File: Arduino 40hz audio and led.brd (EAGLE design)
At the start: 79.2 x 83.2 mm, 28 parts, among them IC1 LM7805, IC2 IRL-Z44N, IC3 LM741

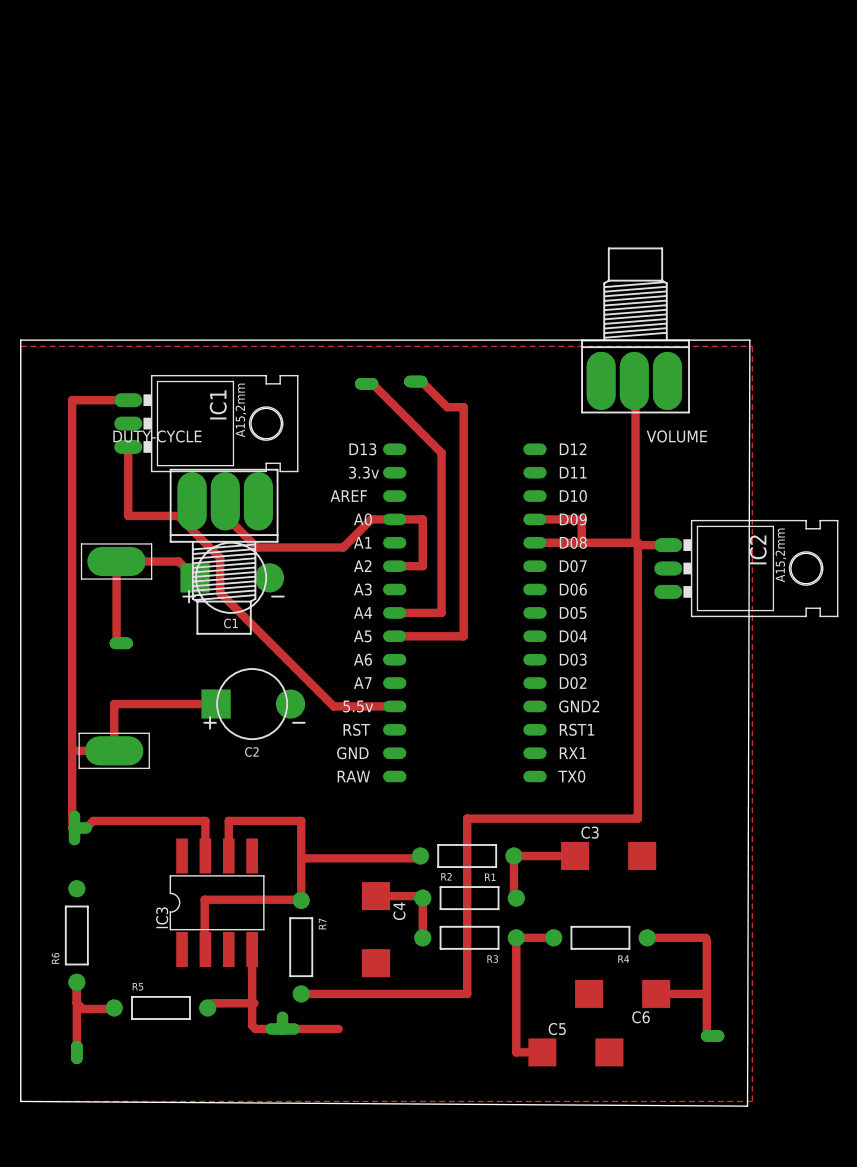
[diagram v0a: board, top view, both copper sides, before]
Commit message: Version 1 is done.. w00t
Version 1 is done.. w00t!!!

Now I need to make some little fixes as I've built the first one.
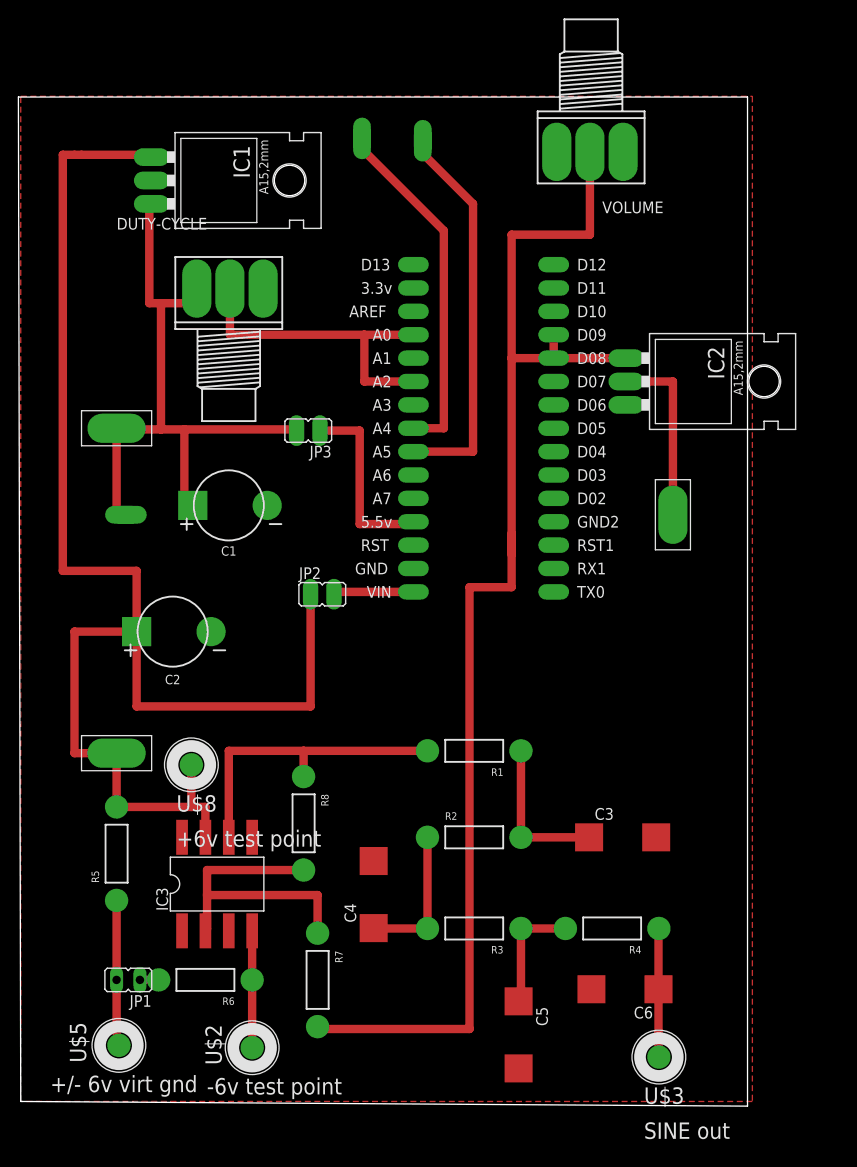
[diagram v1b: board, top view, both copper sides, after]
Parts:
- added JP1: (no value), jumper:JP1
- added JP2, JP3: (no value), jim_muppet_parts:JP1
- added P+3: +6V, jim_muppet_parts:POWER-IN-PAD
- added R8: (no value), jim_muppet_parts:AXIAL-0.4
- U$2: value PAD-2PIN-RECTANGLE -> -6v test point; device jim_muppet_parts:PAD-2PIN-RECTANGLE-50MIL -> jim_muppet_parts:PROBE_POINT_1
- U$3: value PAD-3PIN-RECTANGLE50MIL -> SINE out; device jim_muppet_parts:PAD-3PIN-RECTANGLE-50MIL -> jim_muppet_parts:PROBE_POINT_1
- U$5: value PAD-3PIN-RECTANGLE50MIL -> +/- 6v virt gnd; device jim_muppet_parts:PAD-3PIN-RECTANGLE-50MIL -> jim_muppet_parts:PROBE_POINT_1
- U$8: value PAD-2PIN-RECTANGLE -> +6v test point; device jim_muppet_parts:PAD-2PIN-RECTANGLE-50MIL -> jim_muppet_parts:PROBE_POINT_1
- moved U$2 46.4 mm to (28.7, 3.56)
- moved U$3 45.1 mm to (72.9, 2.54), turned to 0 degrees
- moved U$8 33.0 mm to (22.1, 34.3), turned to 0 degrees
- moved U$5 27.6 mm to (14.2, 3.81), turned to 0 degrees
- moved U$4 26.7 mm to (36.8, 104.9), turned to 90 degrees
- moved IC1 26.5 mm to (17.8, 100.3)
- moved U$6 26.2 mm to (43.4, 104.6), turned to 90 degrees
- moved VOLUME 25.4 mm to (61.7, 104.1)
- moved DUTY-CYCLE 23.1 mm to (22.4, 87.9)
- moved IC2 20.8 mm to (69.3, 78.5)
- moved U$1 20.2 mm to (52.6, 64.5)
- moved R5 17.4 mm to (10.2, 27.2), turned to 90 degrees
- moved R6 14.8 mm to (19.8, 13.5), turned to 180 degrees
- moved P+2 14.5 mm to (10.2, 73.4)
- moved U$7 14.0 mm to (11.2, 64.0)
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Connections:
- removed net N$11: IC3.7, U$5.PAD$3
- removed net N$12: IC3.4, U$3.PAD$3
- new net N$16: JP1.2, R5.P$1, U$5.P$1
- net +12V: now also IC3.7, JP2.1, R5.P$2, U$8.P$1; no longer U$5.PAD$1
- net +5V: now also IC2.GND, JP3.2, P+3.VCC; no longer U$1.5V
- net GND: now also IC3.4, R6.P$1, U$2.P$1; no longer U$3.PAD$1
- net N$10: now also IC3.2, R7.P$1, R8.P$2; no longer R5.P$2, U$3.PAD$2
- net N$13: now also R8.P$1; no longer IC3.2, R7.P$1
- net N$2: now also VOLUME.2
- net N$6: no longer U$2.PAD$1
- net N$7: now also JP1.1; no longer U$5.PAD$2
- net N$8: now also JP2.2, U$1.RAW; no longer IC2.GND, VOLUME.2
- net N$9: now also JP3.1, U$1.5V; no longer R5.P$1, R6.P$1, U$8.PAD$2
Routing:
- net +12V: track 64.9 -> 156.1 mm
- net N$10: track 5.29 -> 33.6 mm
- net N$11: track 26.5 -> 0.00 mm
- net N$2: track 123.8 -> 143.5 mm
- net +5V: track 68.5 -> 86.9 mm
- net N$13: track 49.5 -> 33.8 mm
- net N$16: track 0.00 -> 14.5 mm
- net N$8: track 0.00 -> 8.74 mm
- net N$6: track 22.3 -> 14.8 mm
- net N$5: track 19.3 -> 12.8 mm
- net N$9: track 14.1 -> 20.6 mm
- net N$4: track 9.61 -> 15.8 mm
- net GND: track 19.1 -> 13.2 mm
- net N$3: track 11.5 -> 17.1 mm
- net N$14: track 33.1 -> 37.5 mm
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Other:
- board size 79.2 x 83.2 mm -> 79.2 x 109.7 mm
